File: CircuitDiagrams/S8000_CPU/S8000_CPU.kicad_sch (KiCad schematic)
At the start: 40 parts, among them U1 7404, U101 7404, U103 74244, U104 7404, U11 74240, U12 74244, U122 7404, U127 7404, U13 74113, U14 74113, U15 7402, U16 7451, U17 7400, U18 7402, U2 7410, U20 74113, U21 7432, U22 7432, U23 7410, U27 7432, U29 7404, U3 7408, U30 7410, U32 7404, U33 7411, U34 74260, U35 7407, U38 7408, U4 7421, U41 7432, U42 7408, U5 7408, U54 7427, U56 7432, U6 7402, U61 74260, U7 7474, U8 7432, U81 7414, U9 7400

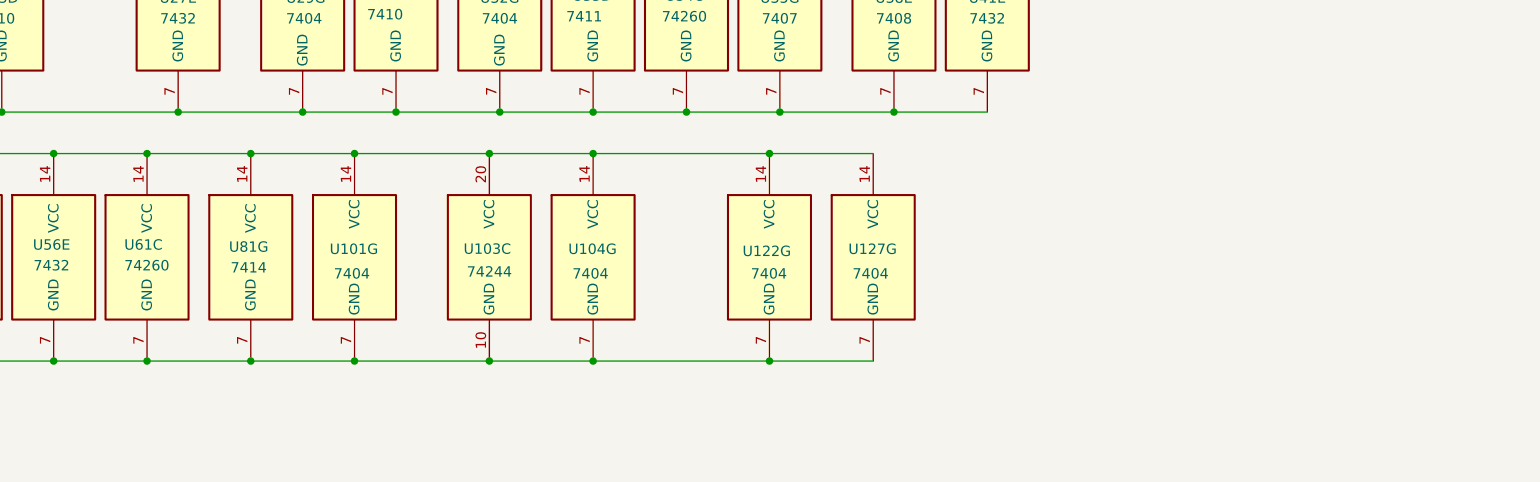
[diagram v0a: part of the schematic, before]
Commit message: page 11 done
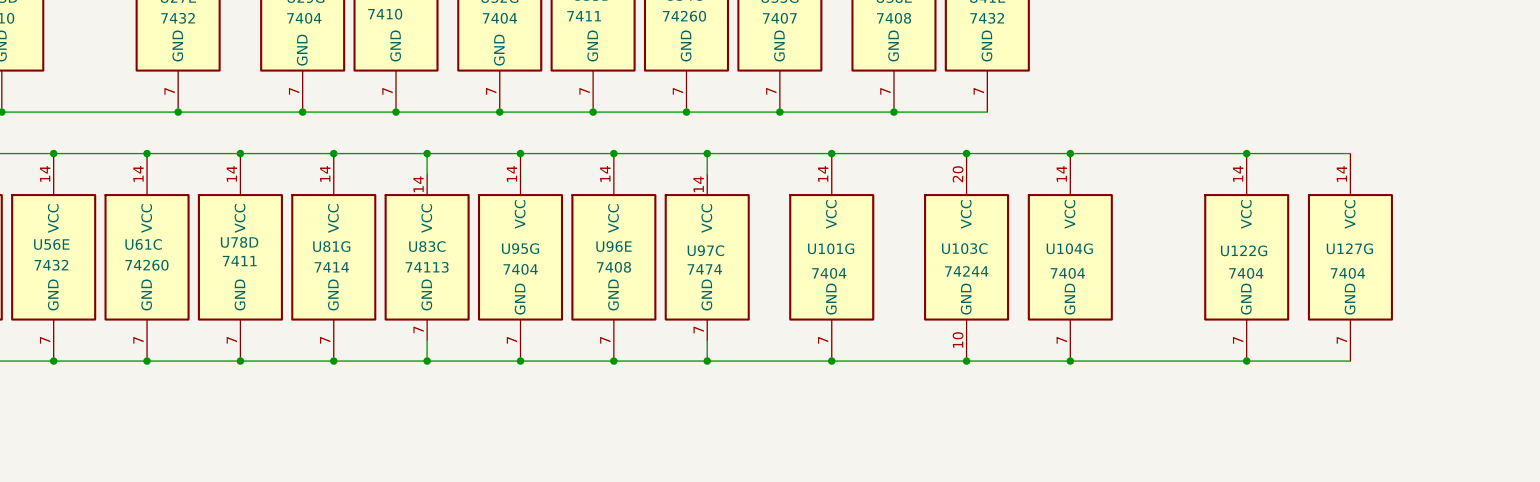
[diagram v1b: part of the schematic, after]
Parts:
- added U78: 7411, symbol 74xx:74LS11
- added U83: 74113, symbol 74xx:74LS113
- added U95: 7404, symbol 74xx:74LS04
- added U96: 7408, symbol 74xx:74LS08
- added U97: 7474, symbol 74xx:74LS74
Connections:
- net +5V: now also U78.14 (VCC), U83.14 (VCC), U95.14 (VCC), U96.14 (VCC), U97.14 (VCC)
- net GND: now also U78.7 (GND), U83.7 (GND), U95.7 (GND), U96.7 (GND), U97.7 (GND)
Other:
- moved on the sheet: U101G, U103C, U104G, U122G, U127G, U81G

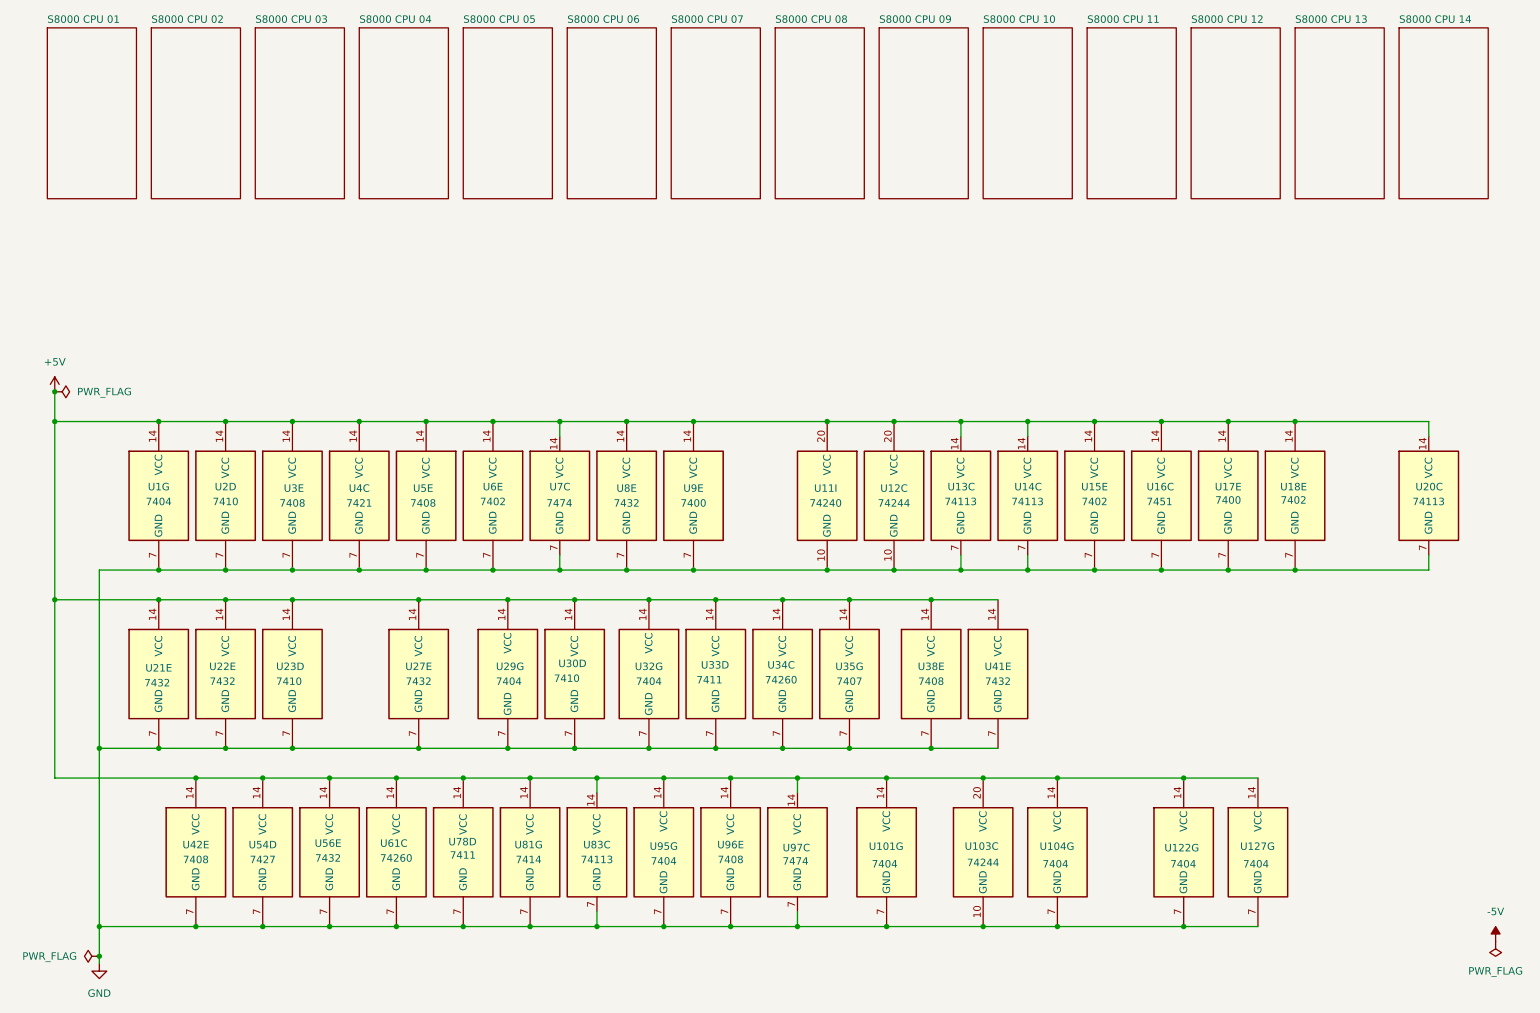
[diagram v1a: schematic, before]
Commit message: page 12 done
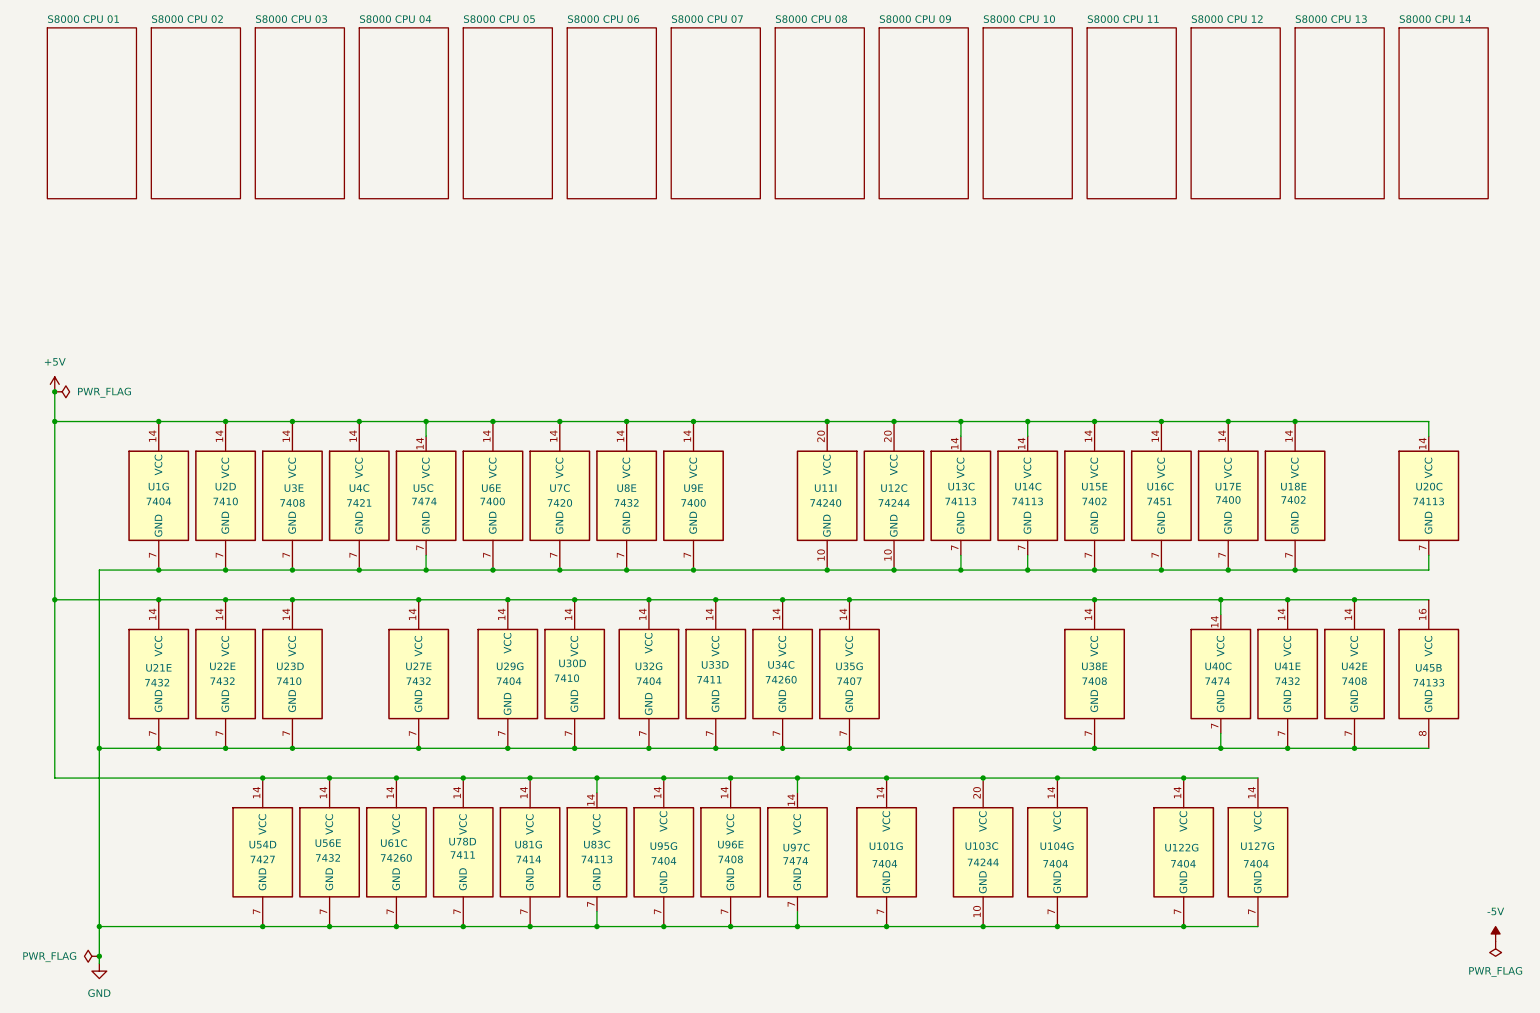
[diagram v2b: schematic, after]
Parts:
- removed U5: 7408, Package_DIP:DIP-14_W7.62mm, symbol 74xx:74LS08
- removed U6: 7402, Package_DIP:DIP-14_W7.62mm, symbol 74xx:74LS02
- removed U7: 7474, symbol 74xx:74LS74
- added U40, U5: 7474, symbol 74xx:74LS74
- added U45: 74133, symbol 74xx:74LS133
- added U6: 7400, symbol 74xx:74LS00
- added U7: 7420, symbol 74xx:74LS20
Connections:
- net +5V: now also U40.14 (VCC), U45.16 (VCC), U5.14 (VCC), U6.14 (VCC), U7.14 (VCC)
- net GND: now also U40.7 (GND), U45.8 (GND), U5.7 (GND), U6.7 (GND), U7.7 (GND)
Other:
- moved on the sheet: U38E, U41E
